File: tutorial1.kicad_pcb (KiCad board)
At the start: 2 copper layers, 5 parts, among them IC1 PIC12C508A-I/SN, J1 MYCONN3

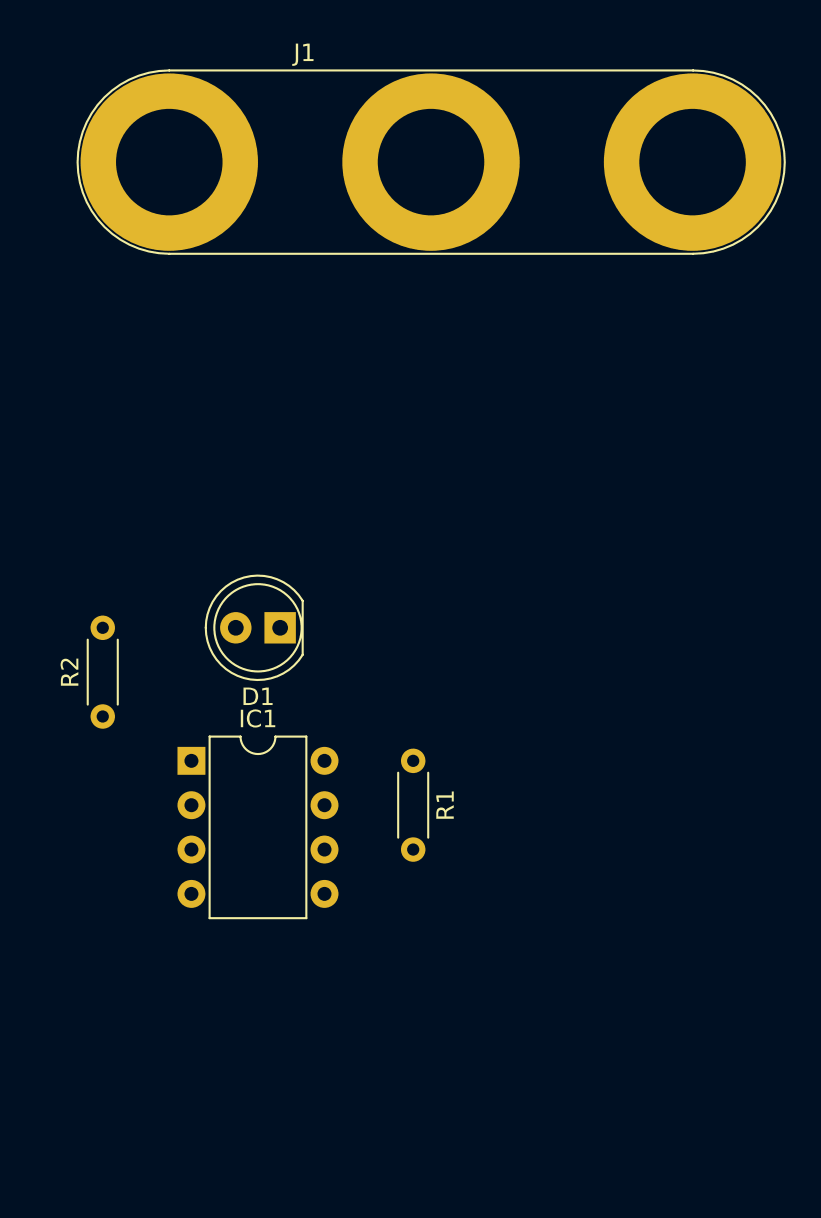
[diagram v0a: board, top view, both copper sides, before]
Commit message: pcb
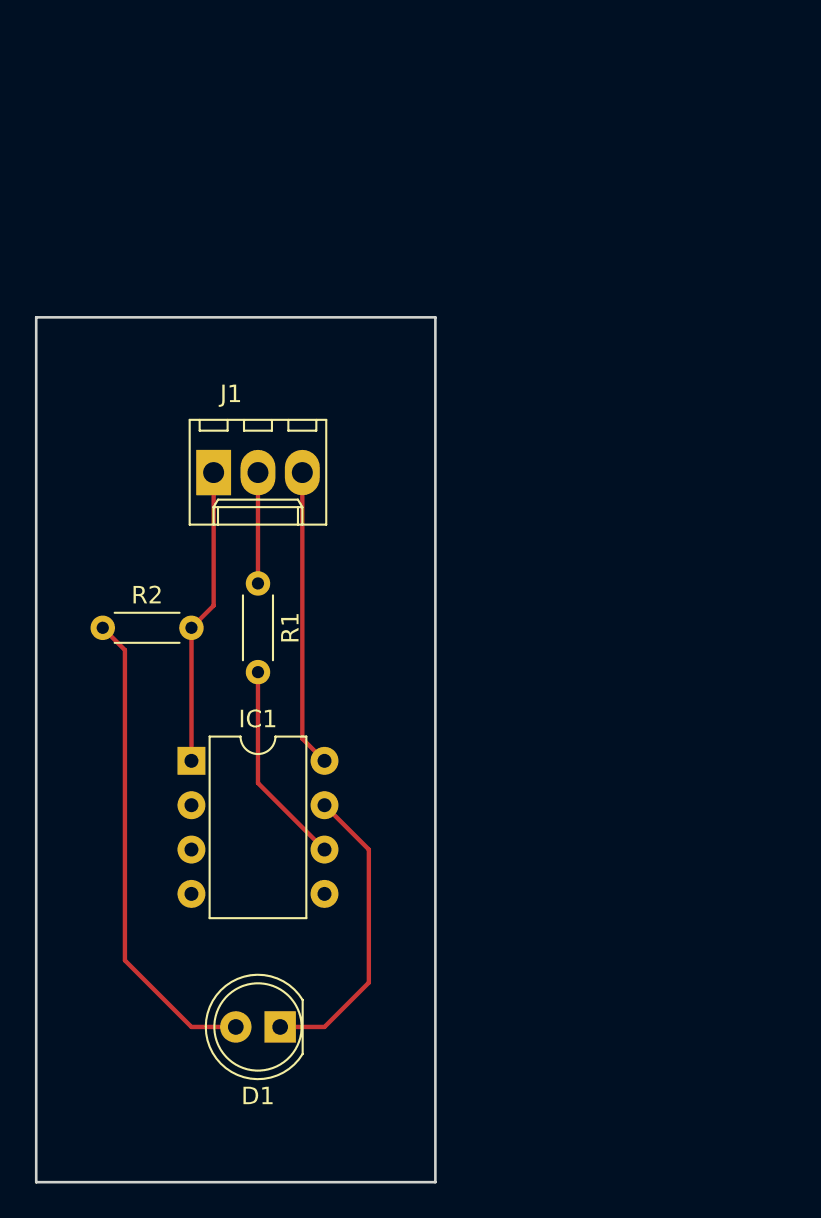
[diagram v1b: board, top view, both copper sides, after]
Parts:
- J1: footprint Connect:Banana_Jack_3Pin -> Connectors_Molex:Molex_KK-6410-03_03x2.54mm_Straight
- moved D1 22.9 mm to (198.1, 106.7)
- moved J1 18.0 mm to (194.3, 74.9)
- moved R1 13.5 mm to (196.8, 81.3)
- moved R2 5.08 mm to (188.0, 83.8), turned to 0 degrees
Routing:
- net Net-(D1-Pad2): track 0.00 -> 27.5 mm
- net /uCtoLED: track 0.00 -> 17.3 mm
- net VCC: track 0.00 -> 17.0 mm
- net GND: track 0.00 -> 17.0 mm
- net /INPUT: track 0.00 -> 11.7 mm
- net /INPUTtoR: track 0.00 -> 6.35 mm
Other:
- board outline added: 22.9 x 49.5 mm
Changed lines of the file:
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@@
   (general
     (links 7)
-    (no_connects 7)
+    (no_connects 0)
     (area 0 0 0 0)
     (thickness 1.6)
-    (drawings 0)
-    (tracks 0)
+    (drawings 4)
+    (tracks 16)
     (zones 0)
     (modules 5)
@@
   )
   (module LEDs:LED_D5.0mm (layer F.Cu)
-    (at 198.12 83.82 180)
+    (at 198.12 106.68 180)
     (descr "LED, diameter 5.0mm, 2 pins, http://cdn-reichelt.de/documents/datenblatt/A500/LL-504BC2E-009.pdf")
     (tags "LED diameter 5.0mm 2 pins")
@@
     )
   )
-  (module Connect:Banana_Jack_3Pin (layer F.Cu)
-    (at 191.77 57.15)
-    (descr "Triple banana socket, footprint - 3 x 6mm drills")
-    (tags "banana socket")
-    (fp_text reference J1 (at 7.75 -6.25) (layer F.SilkS)
-      (effects (font (size 1 1) (thickness 0.15)))
-    )
-    (fp_text value MYCONN3 (at 22.5 -6.25) (layer F.Fab)
-      (effects (font (size 1 1) (thickness 0.15)))
-    )
-    (fp_text user %R (at 14.99 0) (layer F.Fab)
-      (effects (font (size 0.8 0.8) (thickness 0.12)))
-    )
-    (fp_circle (center 30 0) (end 30 -2) (layer F.Fab) (width 0.1))
-    (fp_circle (center 30 0) (end 30 -4.75) (layer F.Fab) (width 0.1))
-    (fp_circle (center 15 0) (end 19.75 0) (layer F.Fab) (width 0.1))
-    (fp_circle (center 15 0) (end 17 0) (layer F.Fab) (width 0.1))
-    (fp_circle (center 0 0) (end 4.75 0) (layer F.Fab) (width 0.1))
-    (fp_circle (center 0 0) (end 2 0) (layer F.Fab) (width 0.1))
-    (fp_line (start 30 5.5) (end 0 5.5) (layer F.CrtYd) (width 0.05))
-    (fp_line (start 0 -5.5) (end 30 -5.5) (layer F.CrtYd) (width 0.05))
-    (fp_arc (start 0 0) (end 0 5.5) (angle 180) (layer F.CrtYd) (width 0.05))
-    (fp_arc (start 30 0) (end 30 -5.5) (angle 180) (layer F.CrtYd) (width 0.05))
-    (fp_line (start 0 5.25) (end 30 5.25) (layer F.SilkS) (width 0.12))
-    (fp_line (start 30 -5.25) (end 0 -5.25) (layer F.SilkS) (width 0.12))
-    (fp_arc (start 30 0) (end 30 -5.25) (angle 180) (layer F.SilkS) (width 0.12))
-    (fp_arc (start 0 0) (end 0 5.25) (angle 180) (layer F.SilkS) (width 0.12))
-    (pad 1 thru_hole circle (at 0 0) (size 10.16 10.16) (drill 6.1) (layers *.Cu *.Mask)
-      (net 3 VCC))
-    (pad 3 thru_hole circle (at 29.97 0) (size 10.16 10.16) (drill 6.1) (layers *.Cu *.Mask)
-      (net 9 GND))
-    (pad 2 thru_hole circle (at 14.99 0) (size 10.16 10.16) (drill 6.1) (layers *.Cu *.Mask)
-      (net 10 /INPUTtoR))
-    (model ${KISYS3DMOD}/Connectors.3dshapes/Banana_Jack_3Pin.wrl
-      (at (xyz 0.5905511811023623 0 0))
-      (scale (xyz 2 2 2))
-      (rotate (xyz 0 0 0))
-    )
-  )
   (module Resistors_ThroughHole:R_Axial_DIN0204_L3.6mm_D1.6mm_P5.08mm_Horizontal (layer F.Cu)
-    (at 205.74 91.44 270)
+    (at 196.85 81.28 270)
     (descr "Resistor, Axial_DIN0204 series, Axial, Horizontal, pin pitch=5.08mm, 0.16666666666666666W = 1/6W, length*diameter=3.6*1.6mm^2, http://cdn-reichelt.de/documents/datenblatt/B400/1_4W%23YAG.pdf")
     (tags "Resistor Axial_DIN0204 series Axial Horizontal pin pitch 5.08mm 0.16666666666666666W = 1/6W length 3.6mm diameter 1.6mm")
@@
   )
   (module Resistors_ThroughHole:R_Axial_DIN0204_L3.6mm_D1.6mm_P5.08mm_Horizontal (layer F.Cu)
-    (at 187.96 88.9 90)
+    (at 187.96 83.82)
     (descr "Resistor, Axial_DIN0204 series, Axial, Horizontal, pin pitch=5.08mm, 0.16666666666666666W = 1/6W, length*diameter=3.6*1.6mm^2, http://cdn-reichelt.de/documents/datenblatt/B400/1_4W%23YAG.pdf")
     (tags "Resistor Axial_DIN0204 series Axial Horizontal pin pitch 5.08mm 0.16666666666666666W = 1/6W length 3.6mm diameter 1.6mm")
-    (fp_text reference R2 (at 2.54 -1.86 90) (layer F.SilkS)
-      (effects (font (size 1 1) (thickness 0.15)))
-    )
-    (fp_text value 1k (at 2.54 1.86 90) (layer F.Fab)
+    (fp_text reference R2 (at 2.54 -1.86) (layer F.SilkS)
+      (effects (font (size 1 1) (thickness 0.15)))
+    )
+    (fp_text value 1k (at 2.54 1.86) (layer F.Fab)
       (effects (font (size 1 1) (thickness 0.15)))
     )
@@
     (fp_line (start 6.05 1.15) (end 6.05 -1.15) (layer F.CrtYd) (width 0.05))
     (fp_line (start 6.05 -1.15) (end -0.95 -1.15) (layer F.CrtYd) (width 0.05))
-    (pad 1 thru_hole circle (at 0 0 90) (size 1.4 1.4) (drill 0.7) (layers *.Cu *.Mask)
+    (pad 1 thru_hole circle (at 0 0) (size 1.4 1.4) (drill 0.7) (layers *.Cu *.Mask)
       (net 2 "Net-(D1-Pad2)"))
-    (pad 2 thru_hole oval (at 5.08 0 90) (size 1.4 1.4) (drill 0.7) (layers *.Cu *.Mask)
+    (pad 2 thru_hole oval (at 5.08 0) (size 1.4 1.4) (drill 0.7) (layers *.Cu *.Mask)
       (net 3 VCC))
     (model ${KISYS3DMOD}/Resistors_THT.3dshapes/R_Axial_DIN0204_L3.6mm_D1.6mm_P5.08mm_Horizontal.wrl
@@
     )
   )
+  (module Connectors_Molex:Molex_KK-6410-03_03x2.54mm_Straight (layer F.Cu)
+    (at 194.31 74.93)
+    (descr "Connector Headers with Friction Lock, 22-27-2031, http://www.molex.com/pdm_docs/sd/022272021_sd.pdf")
+    (tags "connector molex kk_6410 22-27-2031")
+    (fp_text reference J1 (at 1 -4.5) (layer F.SilkS)
+      (effects (font (size 1 1) (thickness 0.15)))
+    )
+    (fp_text value MYCONN3 (at 2.54 4.5) (layer F.Fab)
+      (effects (font (size 1 1) (thickness 0.15)))
+    )
+    (fp_line (start -1.47 -3.12) (end -1.47 3.08) (layer F.Fab) (width 0.12))
+    (fp_line (start -1.47 3.08) (end 6.55 3.08) (layer F.Fab) (width 0.12))
+    (fp_line (start 6.55 3.08) (end 6.55 -3.12) (layer F.Fab) (width 0.12))
+    (fp_line (start 6.55 -3.12) (end -1.47 -3.12) (layer F.Fab) (width 0.12))
+    (fp_line (start -1.37 -3.02) (end -1.37 2.98) (layer F.SilkS) (width 0.12))
+    (fp_line (start -1.37 2.98) (end 6.45 2.98) (layer F.SilkS) (width 0.12))
+    (fp_line (start 6.45 2.98) (end 6.45 -3.02) (layer F.SilkS) (width 0.12))
+    (fp_line (start 6.45 -3.02) (end -1.37 -3.02) (layer F.SilkS) (width 0.12))
+    (fp_line (start 0 2.98) (end 0 1.98) (layer F.SilkS) (width 0.12))
+    (fp_line (start 0 1.98) (end 5.08 1.98) (layer F.SilkS) (width 0.12))
+    (fp_line (start 5.08 1.98) (end 5.08 2.98) (layer F.SilkS) (width 0.12))
+    (fp_line (start 0 1.98) (end 0.25 1.55) (layer F.SilkS) (width 0.12))
+    (fp_line (start 0.25 1.55) (end 4.83 1.55) (layer F.SilkS) (width 0.12))
+    (fp_line (start 4.83 1.55) (end 5.08 1.98) (layer F.SilkS) (width 0.12))
+    (fp_line (start 0.25 2.98) (end 0.25 1.98) (layer F.SilkS) (width 0.12))
+    (fp_line (start 4.83 2.98) (end 4.83 1.98) (layer F.SilkS) (width 0.12))
+    (fp_line (start -0.8 -3.02) (end -0.8 -2.4) (layer F.SilkS) (width 0.12))
+    (fp_line (start -0.8 -2.4) (end 0.8 -2.4) (layer F.SilkS) (width 0.12))
+    (fp_line (start 0.8 -2.4) (end 0.8 -3.02) (layer F.SilkS) (width 0.12))
+    (fp_line (start 1.74 -3.02) (end 1.74 -2.4) (layer F.SilkS) (width 0.12))
+    (fp_line (start 1.74 -2.4) (end 3.34 -2.4) (layer F.SilkS) (width 0.12))
+    (fp_line (start 3.34 -2.4) (end 3.34 -3.02) (layer F.SilkS) (width 0.12))
+    (fp_line (start 4.28 -3.02) (end 4.28 -2.4) (layer F.SilkS) (width 0.12))
+    (fp_line (start 4.28 -2.4) (end 5.88 -2.4) (layer F.SilkS) (width 0.12))
+    (fp_line (start 5.88 -2.4) (end 5.88 -3.02) (layer F.SilkS) (width 0.12))
+    (fp_line (start -1.9 3.5) (end -1.9 -3.55) (layer F.CrtYd) (width 0.05))
+    (fp_line (start -1.9 -3.55) (end 7 -3.55) (layer F.CrtYd) (width 0.05))
+    (fp_line (start 7 -3.55) (end 7 3.5) (layer F.CrtYd) (width 0.05))
+    (fp_line (start 7 3.5) (end -1.9 3.5) (layer F.CrtYd) (width 0.05))
+    (fp_text user %R (at 2.54 0) (layer F.Fab)
+      (effects (font (size 1 1) (thickness 0.15)))
+    )
+    (pad 1 thru_hole rect (at 0 0) (size 2 2.6) (drill 1.2) (layers *.Cu *.Mask)
+      (net 3 VCC))
+    (pad 2 thru_hole oval (at 2.54 0) (size 2 2.6) (drill 1.2) (layers *.Cu *.Mask)
+      (net 10 /INPUTtoR))
+    (pad 3 thru_hole oval (at 5.08 0) (size 2 2.6) (drill 1.2) (layers *.Cu *.Mask)
+      (net 9 GND))
+    (model ${KISYS3DMOD}/Connectors_Molex.3dshapes/Molex_KK-6410-03_03x2.54mm_Straight.wrl
+      (at (xyz 0 0 0))
+      (scale (xyz 1 1 1))
+      (rotate (xyz 0 0 0))
+    )
+  )
+  (gr_line (start 207.01 66.04) (end 184.15 66.04) (angle 90) (layer Edge.Cuts) (width 0.15))
+  (gr_line (start 207.01 115.57) (end 207.01 66.04) (angle 90) (layer Edge.Cuts) (width 0.15))
+  (gr_line (start 184.15 115.57) (end 207.01 115.57) (angle 90) (layer Edge.Cuts) (width 0.15))
+  (gr_line (start 184.15 66.04) (end 184.15 115.57) (angle 90) (layer Edge.Cuts) (width 0.15))
+  (segment (start 198.12 106.68) (end 200.66 106.68) (width 0.25) (layer F.Cu) (net 1) (status 400000))
+  (segment (start 203.2 96.52) (end 200.66 93.98) (width 0.25) (layer F.Cu) (net 1) (status 800000))
+  (segment (start 203.2 104.14) (end 203.2 96.52) (width 0.25) (layer F.Cu) (net 1))
+  (segment (start 200.66 106.68) (end 203.2 104.14) (width 0.25) (layer F.Cu) (net 1))
+  (segment (start 195.58 106.68) (end 193.04 106.68) (width 0.25) (layer F.Cu) (net 2) (status 400000))
+  (segment (start 189.23 85.09) (end 187.96 83.82) (width 0.25) (layer F.Cu) (net 2) (status 800000))
+  (segment (start 189.23 102.87) (end 189.23 85.09) (width 0.25) (layer F.Cu) (net 2))
+  (segment (start 193.04 106.68) (end 189.23 102.87) (width 0.25) (layer F.Cu) (net 2))
+  (segment (start 193.04 91.44) (end 193.04 83.82) (width 0.25) (layer F.Cu) (net 3) (status C00000))
+  (segment (start 194.31 74.93) (end 194.31 82.55) (width 0.25) (layer F.Cu) (net 3) (status 400000))
+  (segment (start 194.31 82.55) (end 193.04 83.82) (width 0.25) (layer F.Cu) (net 3) (status 800000))
+  (segment (start 196.85 86.36) (end 196.85 92.71) (width 0.25) (layer F.Cu) (net 6) (status 400000))
+  (segment (start 196.85 92.71) (end 200.66 96.52) (width 0.25) (layer F.Cu) (net 6) (status 800000))
+  (segment (start 199.39 74.93) (end 199.39 90.17) (width 0.25) (layer F.Cu) (net 9) (status 400000))
+  (segment (start 199.39 90.17) (end 200.66 91.44) (width 0.25) (layer F.Cu) (net 9) (status 800000))
+  (segment (start 196.85 74.93) (end 196.85 81.28) (width 0.25) (layer F.Cu) (net 10) (status C00000))
 )
